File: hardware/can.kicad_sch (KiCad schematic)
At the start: 10 parts, among them U2 MCP2542FDxMF

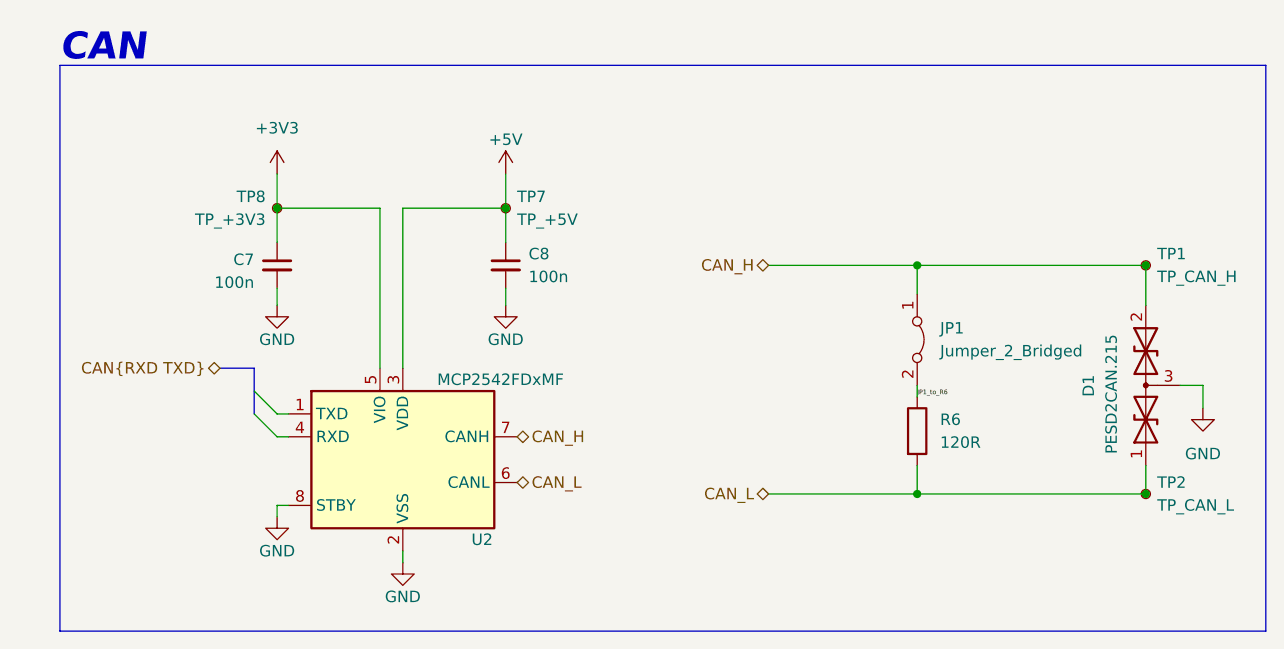
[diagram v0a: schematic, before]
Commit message: Poprawione busy, brak errorow
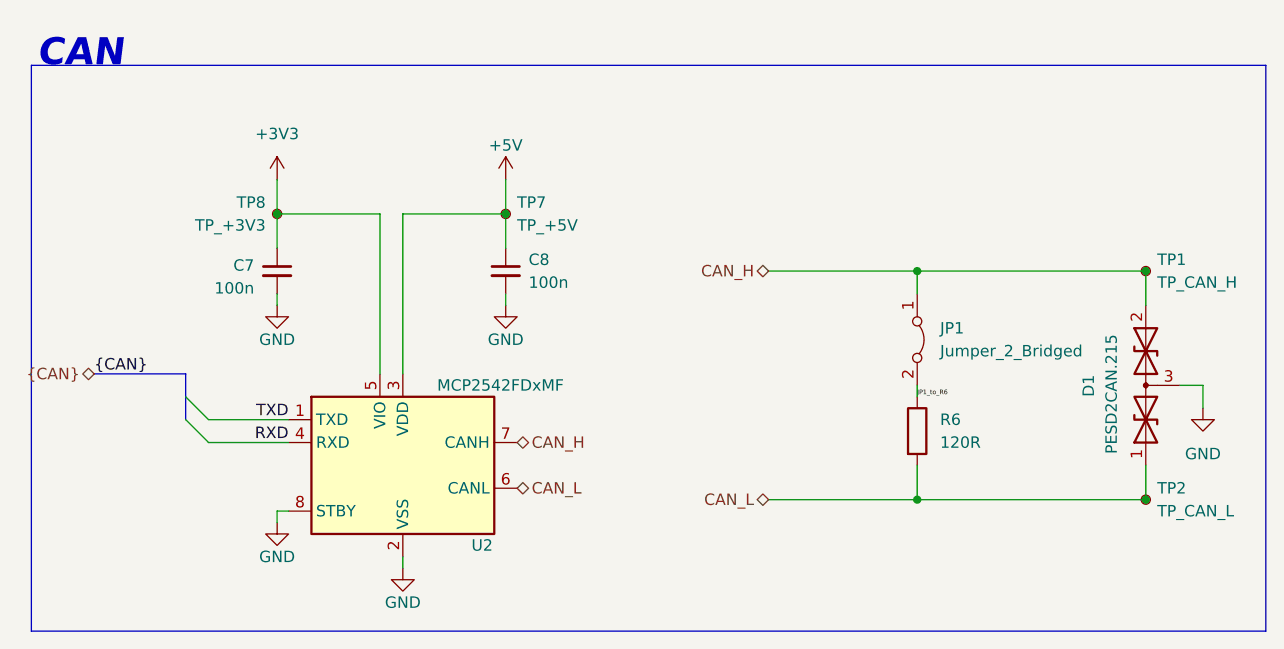
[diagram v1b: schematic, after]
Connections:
- net TXD: now reaches U2.1 (TXD)
- net RXD: now reaches U2.4 (RXD)
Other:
- moved on the sheet: C7, C8, TP1, TP2, TP7, TP8, U2
